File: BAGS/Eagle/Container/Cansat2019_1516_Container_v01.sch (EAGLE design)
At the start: 27 parts, among them IC1 LM1117-3.3V-SOT223, IC2 24C64SM, Q1 MOSFET-NCHANNEL2N7000, Q2 TIP120, U1 TINY45-20-DIP

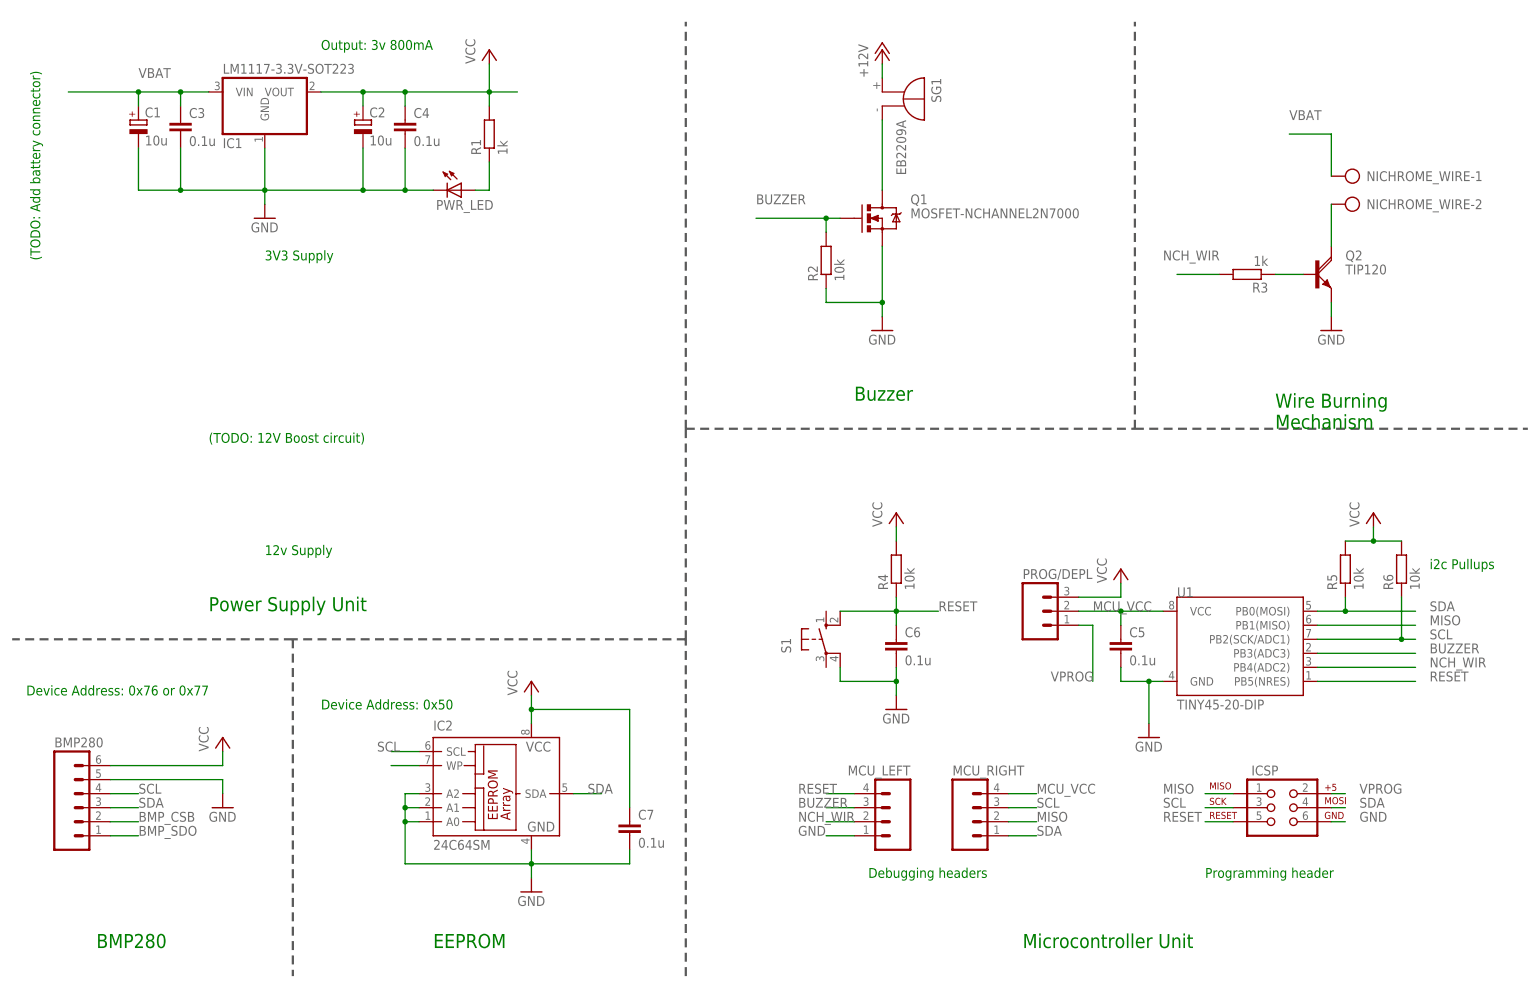
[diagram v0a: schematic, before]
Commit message: Add files via upload
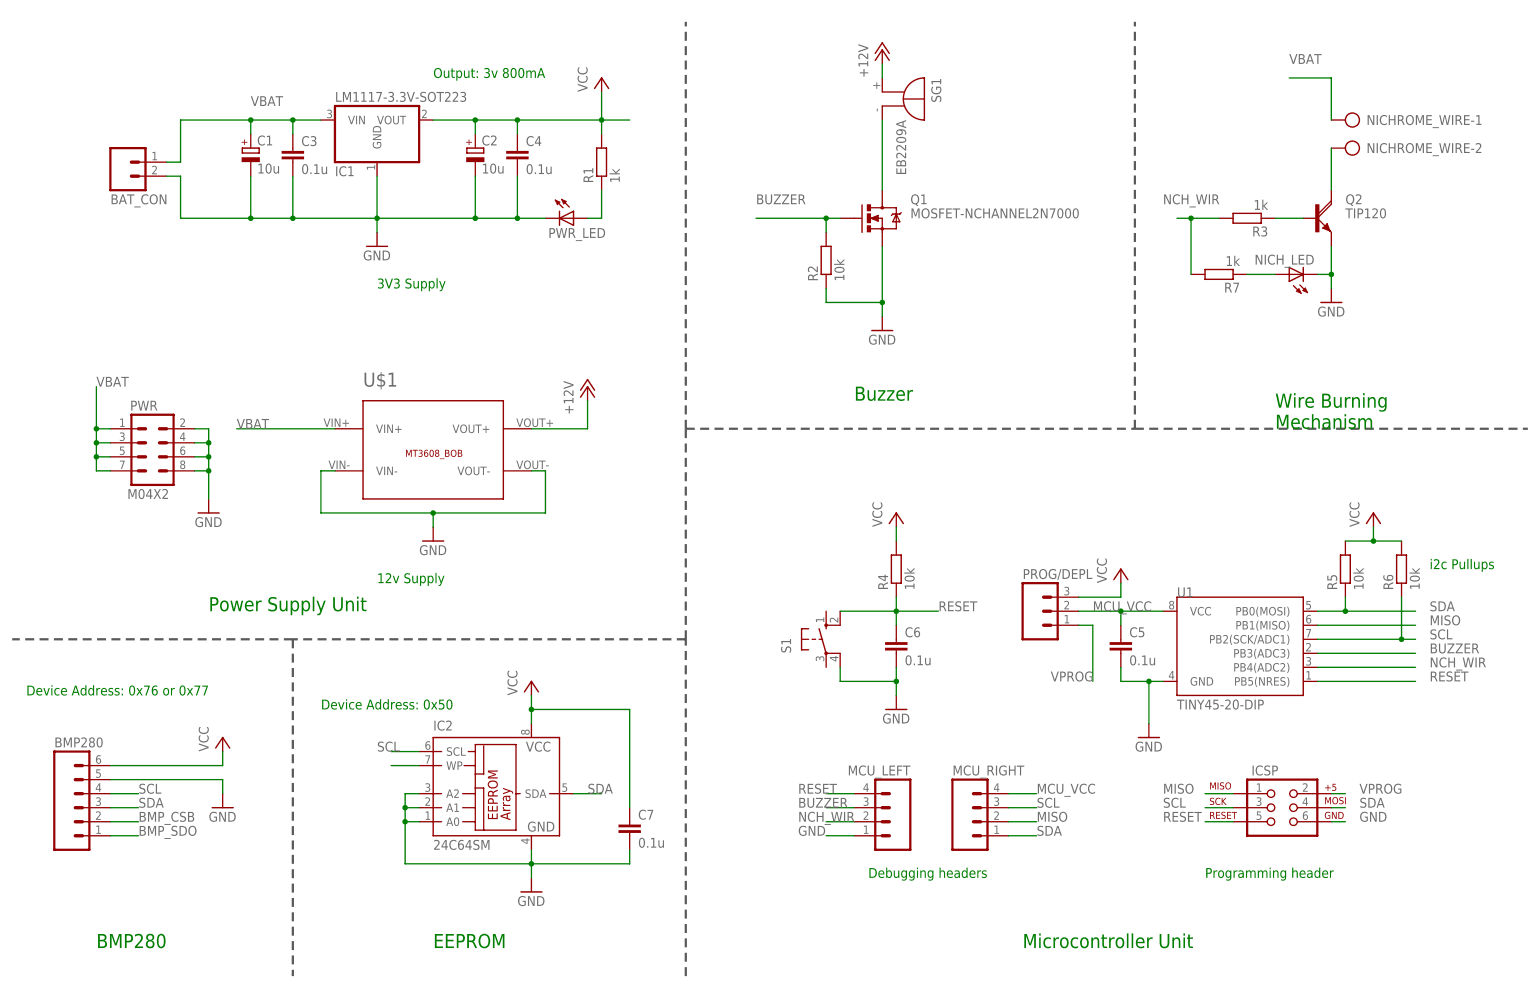
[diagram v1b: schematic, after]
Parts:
- added BAT_CON: (no value), CEDT_JANUARY_2015_v5:M02
- added NICH_LED: (no value), 01_adafruit:LED3MM
- added PWR: M04X2, SparkFun-Connectors:M04X2
- added R7: 1k, rcl:R-EU_0204/7
- added U$1: MT3608_BOB, Breakouts:MT3608_BOB
- MCU_LEFT, MCU_RIGHT: device SparkFun-Connectors:M04PTH -> con-amp-quick:M04
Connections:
- new net N$5: NICH_LED.A, R7.1
- net +12V: now also U$1.VOUT+
- net GND: now also BAT_CON.2, NICH_LED.C, PWR.2, PWR.4, PWR.6, PWR.8, U$1.VIN-, U$1.VOUT-
- net NCH_WIR: now also R7.2
- net VBAT: now also BAT_CON.1, PWR.1, PWR.3, PWR.5, PWR.7, U$1.VIN+
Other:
- note removed: "(TODO: 12V Boost circuit)"
- note removed: "(TODO: Add battery connector)"
- moved on the sheet: C1, C2, C3, C4, IC1, NICHROME_WIRE-1, NICHROME_WIRE-2, PWR_LED, Q2, R1, R3
